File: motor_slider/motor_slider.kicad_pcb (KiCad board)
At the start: 2 copper layers, 60 x 47 mm, 90 parts, among them J1 USB_C_Receptacle_USB2.0_16P, J2 Conn_02x02_Odd_Even, J6 VM, J7 GND, J8 Conn_01x03, SW1 BOOT, SW2 RESET, U1 DRV8833PWP, U10 MOTOR6, U11 DRV8833PWP, U12 MOTOR7, U13 MOTOR8, U14 POT1, U15 DRV8833PWP, U16 ME6210A33M3G, U17 POT2, U18 POT3, U19 POT4, U2 MOTOR1, U20 POT5, U21 POT6, U22 SWD, U23 POT7, U24 POT8, U3 CH32V203C8T6, U4 ME6210A33M3G, U5 MOTOR2, U6 MOTOR3, U7 MOTOR4, U8 DRV8833PWP, U9 MOTOR5, Y1 8M

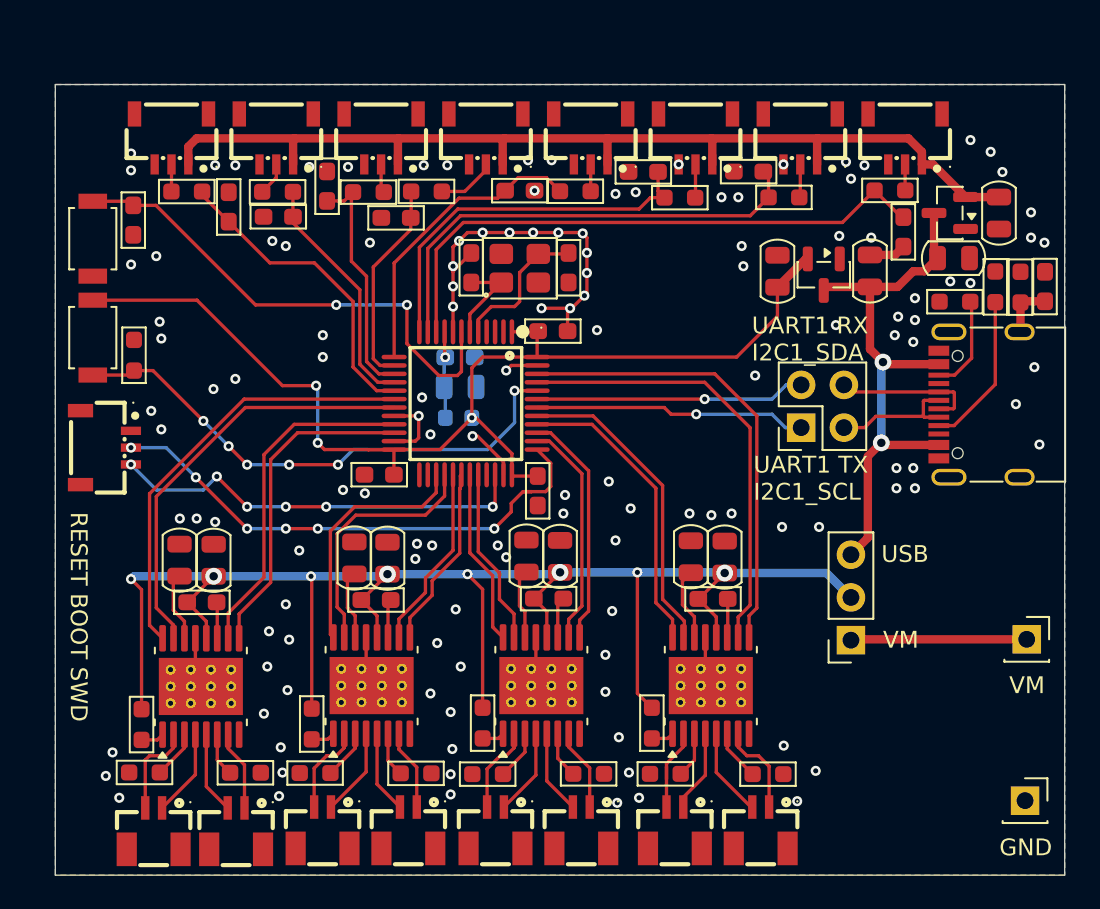
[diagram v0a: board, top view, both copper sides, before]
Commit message: refactor: 更新硬件pcb
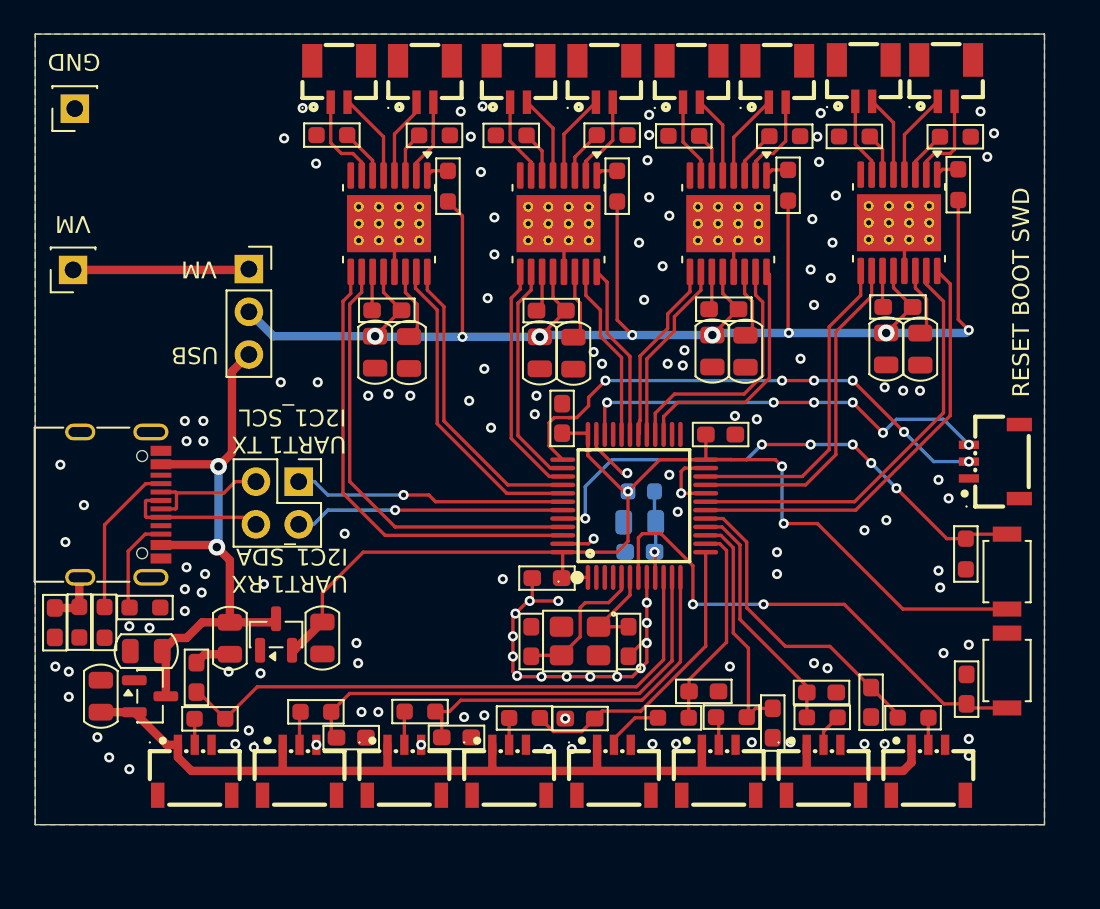
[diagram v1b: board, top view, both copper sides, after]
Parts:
- moved J7 69.9 mm to (69.5, 47.0), turned to 180 degrees
- moved U2 64.8 mm to (121.3, 45.4), turned to 0 degrees
- moved C4 62.2 mm to (68.3, 77.6), turned to -90 degrees
- moved R5 61.2 mm to (121.8, 48.7), turned to 0 degrees
- moved J6 60.8 mm to (69.4, 56.6), turned to 180 degrees
- moved C20 60.6 mm to (71.0, 82.0), turned to -90 degrees
- moved SW2 59.8 mm to (124.9, 80.1), turned to -90 degrees
- moved R4 59.4 mm to (69.7, 77.6), turned to -90 degrees
- moved U24 58.6 mm to (120.2, 86.3), turned to 0 degrees
- moved R7 58.2 mm to (122.0, 51.6), turned to -90 degrees
- moved U5 58.0 mm to (116.4, 45.4), turned to 0 degrees
- moved C1 56.8 mm to (122.5, 81.5), turned to 90 degrees
- moved R2 56.6 mm to (71.2, 77.6), turned to -90 degrees
- moved U14 56.5 mm to (76.6, 86.3), turned to 0 degrees
- moved SW1 55.9 mm to (124.9, 74.2), turned to -90 degrees
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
